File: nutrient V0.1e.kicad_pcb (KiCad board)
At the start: 2 copper layers, 99.1 x 71.1 mm, 76 parts, among them J1 Conn_01x04_Female, J10 Conn_01x01_Male, J2 Conn_01x04_Female, J3 Conn_01x04_Female, J4 Conn_01x04_Female, J5 Conn_01x04_Female, J6 Conn_01x04_Female, J7 Conn_01x03_Male, J8 Conn_01x03_Male, J9 Conn_01x01_Male, P1 SolderJumper_2_Open, P2 SolderJumper_2_Bridged, Q1 Q_NMOS_DGS, Q10 Q_NMOS_DGS, Q2 Q_NMOS_DGS, Q3 Q_NMOS_DGS, Q4 Q_NMOS_DGS, Q5 Q_NMOS_DGS, Q6 Q_NMOS_DGS, Q7 Q_NMOS_DGS, Q8 2N3904, U1 23LC512, U2 DS1307+, Y1 Crystal_Small

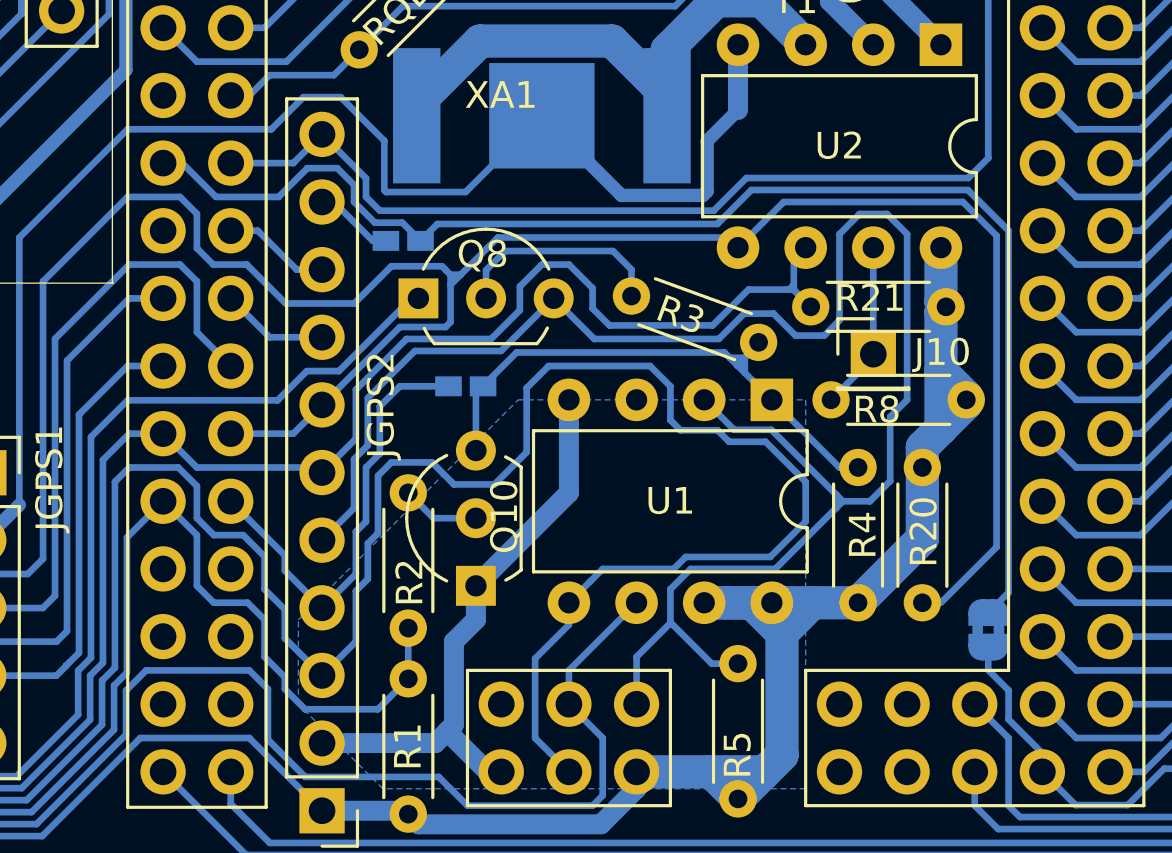
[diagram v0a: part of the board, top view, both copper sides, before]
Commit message: Minor layout change
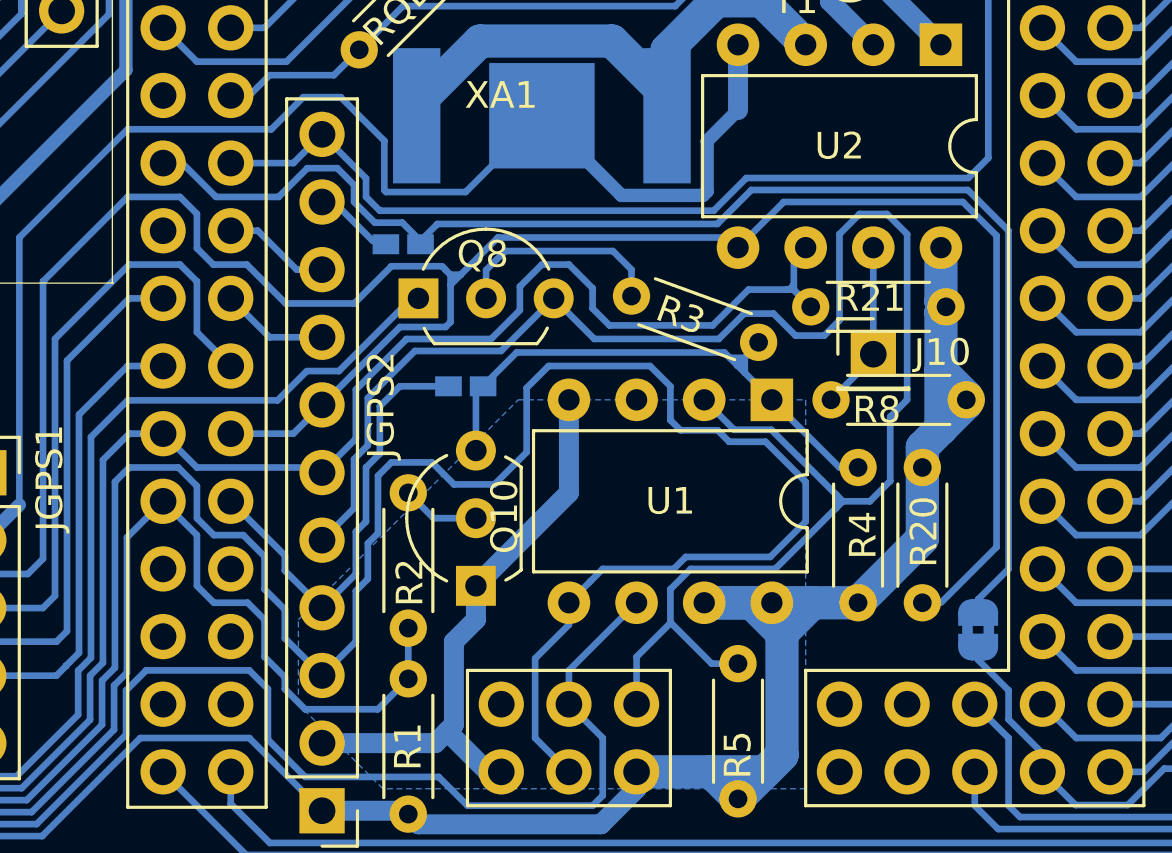
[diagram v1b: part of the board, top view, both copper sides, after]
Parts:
- moved P2 0.38 mm to (152.5, 96.3)
- moved P1 0.13 mm to (130.9, 81.8)
